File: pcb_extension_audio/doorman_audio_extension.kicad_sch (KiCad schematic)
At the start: 36 parts, among them J1 Audio Out, J2 GPIO, J4 Extension Board Connector, J5 Audio In, U1 ES8388

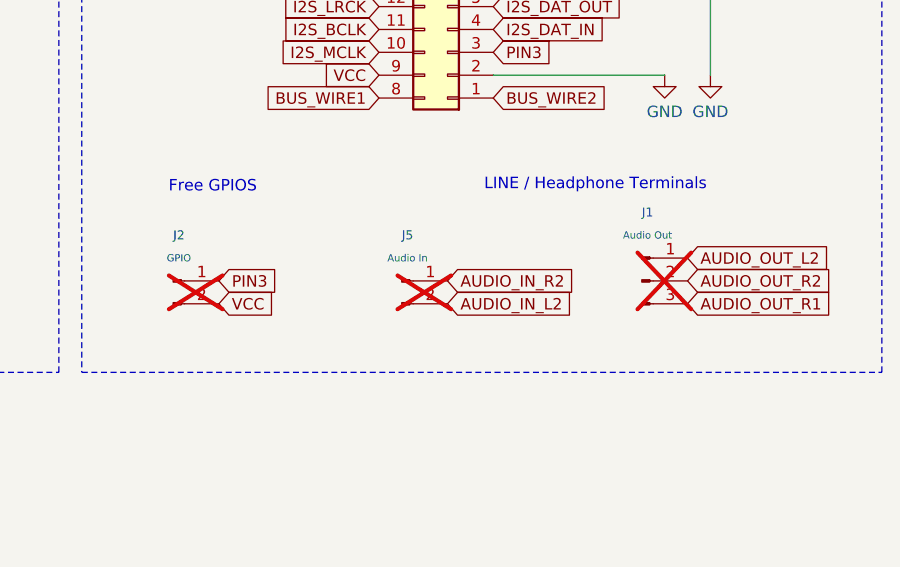
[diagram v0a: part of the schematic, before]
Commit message: WIP
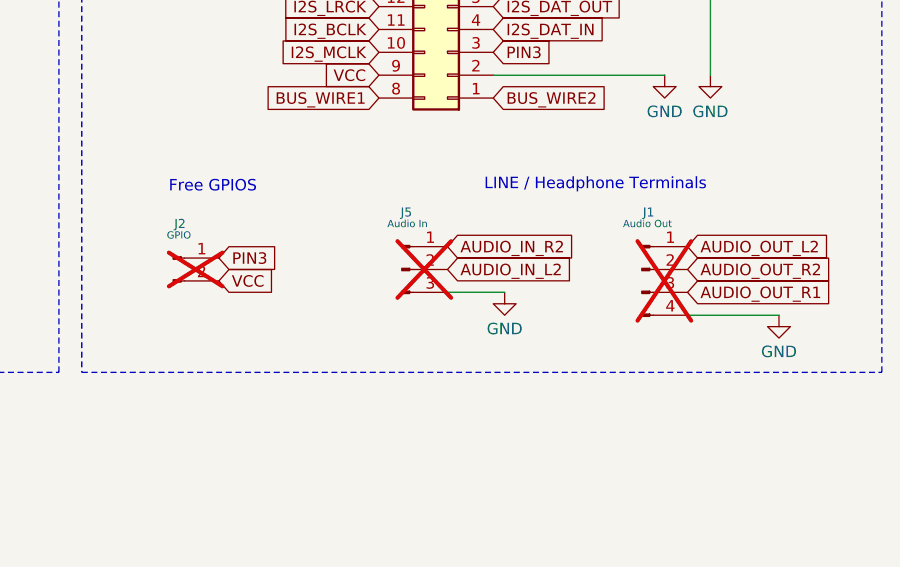
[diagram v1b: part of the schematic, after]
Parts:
- J1: footprint Connector_PinHeader_2.54mm:PinHeader_1x03_P2.54mm_Vertical -> Connector_PinHeader_2.54mm:PinHeader_1x04_P2.54mm_Vertical; symbol Connector:Conn_01x03_Pin -> Connector:Conn_01x04_Pin
- J5: footprint Connector_PinHeader_2.54mm:PinHeader_1x02_P2.54mm_Vertical -> Connector_PinHeader_2.54mm:PinHeader_1x03_P2.54mm_Vertical; symbol Connector:Conn_01x02_Pin -> Connector:Conn_01x03_Pin
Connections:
- net GND: now also J1.4 (Pin_4), J5.3 (Pin_3)
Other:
- moved on the sheet: J2
